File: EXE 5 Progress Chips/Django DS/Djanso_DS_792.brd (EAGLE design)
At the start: 28.9 x 21.9 mm, 1 part

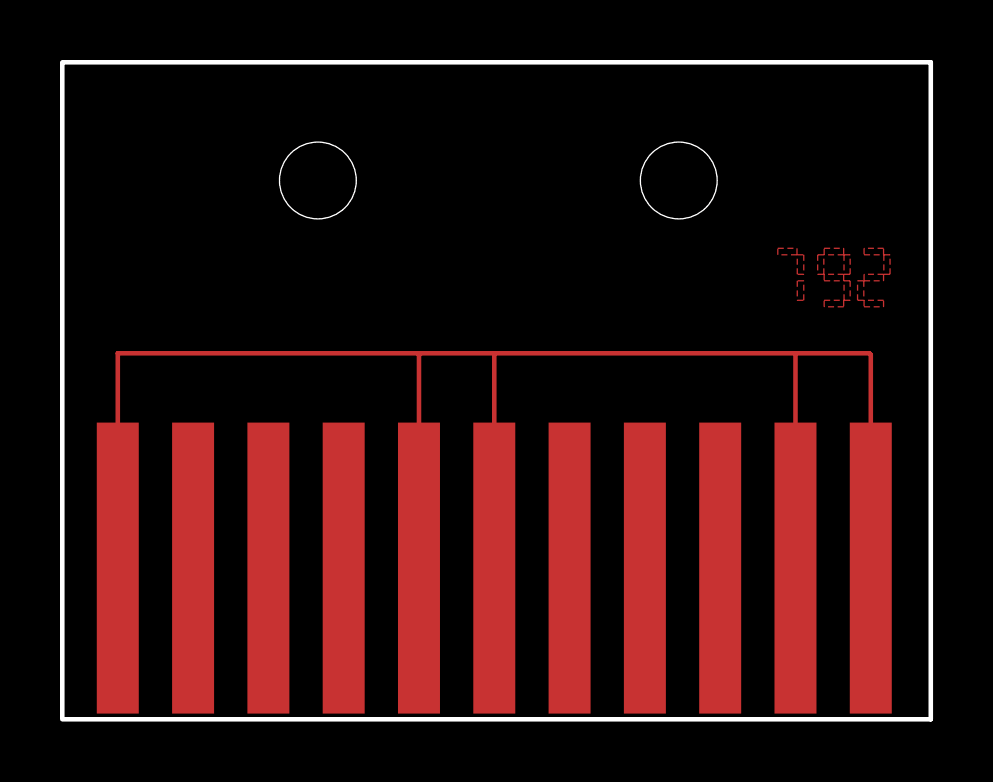
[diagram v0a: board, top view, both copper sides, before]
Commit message: Replace Djanso_DS_792.brd
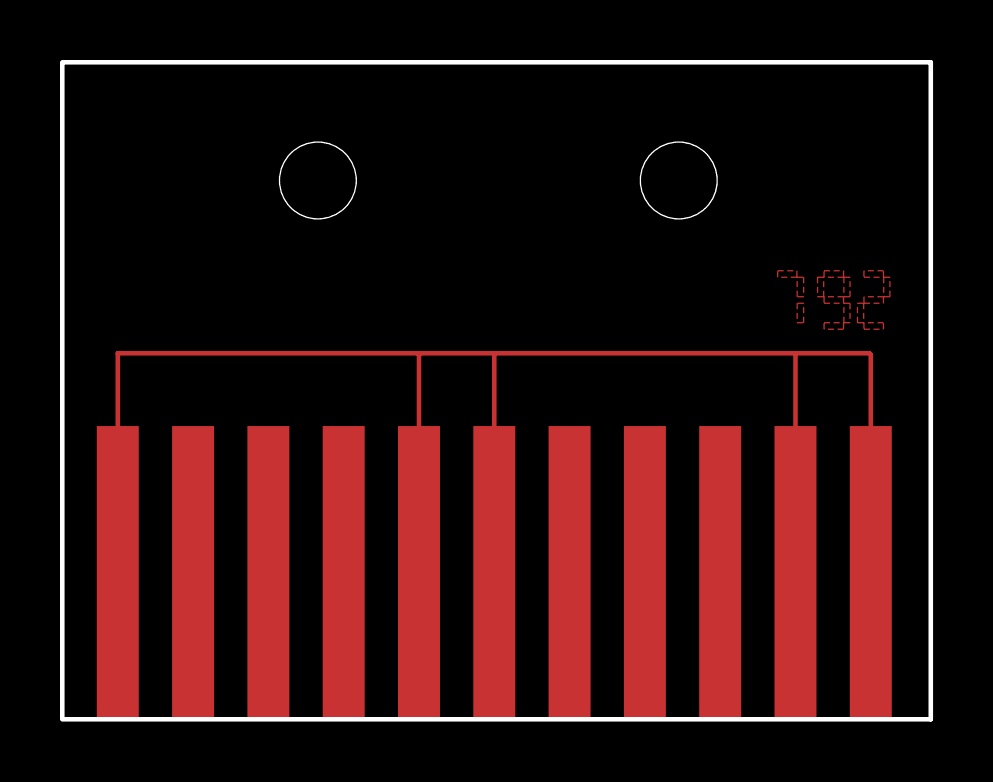
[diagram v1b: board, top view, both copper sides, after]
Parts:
- moved U$1 0.12 mm to (67.3, 20.2)
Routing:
- net N$1: track 60.9 -> 61.5 mm
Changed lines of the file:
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@@
 <setting verticaltext="up"/>
 </settings>
-<grid distance="1" unitdist="mic" unit="mic" style="lines" multiple="1" display="no" altdistance="1" altunitdist="mm" altunit="mm"/>
+<grid distance="1" unitdist="mic" unit="mm" style="lines" multiple="1" display="no" altdistance="1" altunitdist="mm" altunit="mm"/>
 <layers>
 <layer number="1" name="Top" color="4" fill="1" visible="yes" active="yes"/>
@@
 </autorouter>
 <elements>
-<element name="U$1" library="advpins" package="ADCHIP" value="ADVCHIP" x="67.31" y="20.32" smashed="yes"/>
+<element name="U$1" library="advpins" package="ADCHIP" value="ADVCHIP" x="67.31" y="20.205" smashed="yes"/>
 </elements>
 <signals>
@@
 <contactref element="U$1" pad="P$11"/>
 <contactref element="U$1" pad="P$6"/>
-<wire x1="39.7" y1="25.34" x2="39.7" y2="32.5" width="0.1524" layer="1"/>
+<wire x1="39.7" y1="25.225" x2="39.7" y2="32.5" width="0.1524" layer="1"/>
 <wire x1="39.7" y1="32.5" x2="49.8" y2="32.5" width="0.1524" layer="1"/>
 <wire x1="49.8" y1="32.5" x2="52.25" y2="32.5" width="0.1524" layer="1"/>
 <wire x1="52.25" y1="32.5" x2="62.3" y2="32.5" width="0.1524" layer="1"/>
 <wire x1="64.75" y1="32.5" x2="62.3" y2="32.5" width="0.1524" layer="1"/>
-<wire x1="49.74" y1="25.34" x2="49.74" y2="32.44" width="0.1524" layer="1"/>
+<wire x1="49.74" y1="25.225" x2="49.74" y2="32.44" width="0.1524" layer="1"/>
 <wire x1="49.74" y1="32.44" x2="49.8" y2="32.5" width="0.1524" layer="1"/>
-<wire x1="52.25" y1="25.34" x2="52.25" y2="32.5" width="0.1524" layer="1"/>
-<wire x1="62.29" y1="25.34" x2="62.29" y2="32.49" width="0.1524" layer="1"/>
+<wire x1="52.25" y1="25.225" x2="52.25" y2="32.5" width="0.1524" layer="1"/>
+<wire x1="62.29" y1="25.225" x2="62.29" y2="32.49" width="0.1524" layer="1"/>
 <wire x1="62.29" y1="32.49" x2="62.3" y2="32.5" width="0.1524" layer="1"/>
-<wire x1="64.8" y1="25.34" x2="64.8" y2="32.45" width="0.1524" layer="1"/>
+<wire x1="64.8" y1="25.225" x2="64.8" y2="32.45" width="0.1524" layer="1"/>
 <wire x1="64.8" y1="32.45" x2="64.75" y2="32.5" width="0.1524" layer="1"/>
 </signal>
 <signal name="N$4">
-<polygon width="0.001" layer="1">
-<vertex x="62.56625" y="35.132809375"/>
-<vertex x="62.349690625" y="35.132809375"/>
-<vertex x="62.349690625" y="35.7825"/>
-<vertex x="62.56625" y="35.7825"/>
+<polygon width="0.001" layer="1" rank="4">
+<vertex x="62.56225" y="34.384809375"/>
+<vertex x="62.345690625" y="34.384809375"/>
+<vertex x="62.345690625" y="35.0345"/>
+<vertex x="62.56225" y="35.0345"/>
 </polygon>
 </signal>
 <signal name="N$2">
-<polygon width="0.001" layer="1">
-<vertex x="62.340690625" y="35.7825"/>
-<vertex x="61.7" y="35.7825"/>
-<vertex x="61.7" y="35.999059375"/>
-<vertex x="62.340690625" y="35.999059375"/>
+<polygon width="0.001" layer="1" rank="4">
+<vertex x="62.336690625" y="35.0345"/>
+<vertex x="61.696" y="35.0345"/>
+<vertex x="61.696" y="35.251059375"/>
+<vertex x="62.336690625" y="35.251059375"/>
 </polygon>
 </signal>
 <signal name="N$3">
-<polygon width="0.001" layer="1">
-<vertex x="62.349690625" y="34.91625"/>
-<vertex x="62.349690625" y="34.266559375"/>
-<vertex x="62.56625" y="34.266559375"/>
-<vertex x="62.56625" y="34.91625"/>
+<polygon width="0.001" layer="1" rank="4">
+<vertex x="62.345690625" y="34.16825"/>
+<vertex x="62.345690625" y="33.518559375"/>
+<vertex x="62.56225" y="33.518559375"/>
+<vertex x="62.56225" y="34.16825"/>
 </polygon>
 </signal>
 <signal name="N$10">
-<polygon width="0.001" layer="1">
-<vertex x="63.246259375" y="35.132809375"/>
-<vertex x="63.246259375" y="34.91625"/>
-<vertex x="63.895940625" y="34.91625"/>
-<vertex x="63.895940625" y="35.132809375"/>
+<polygon width="0.001" layer="1" rank="4">
+<vertex x="63.242259375" y="34.384809375"/>
+<vertex x="63.242259375" y="34.16825"/>
+<vertex x="63.891940625" y="34.16825"/>
+<vertex x="63.891940625" y="34.384809375"/>
 </polygon>
 </signal>
 <signal name="N$14">
-<polygon width="0.001" layer="1">
-<vertex x="63.895940625" y="34.05"/>
-<vertex x="63.246259375" y="34.05"/>
-<vertex x="63.246259375" y="34.266559375"/>
-<vertex x="63.895940625" y="34.266559375"/>
+<polygon width="0.001" layer="1" rank="4">
+<vertex x="63.891940625" y="33.302"/>
+<vertex x="63.242259375" y="33.302"/>
+<vertex x="63.242259375" y="33.518559375"/>
+<vertex x="63.891940625" y="33.518559375"/>
 </polygon>
 </signal>
 <signal name="N$9">
-<polygon width="0.001" layer="1">
-<vertex x="64.112509375" y="34.266559375"/>
-<vertex x="63.907940625" y="34.266559375"/>
-<vertex x="63.907940625" y="34.91625"/>
-<vertex x="64.112509375" y="34.91625"/>
+<polygon width="0.001" layer="1" rank="4">
+<vertex x="64.108509375" y="33.518559375"/>
+<vertex x="63.903940625" y="33.518559375"/>
+<vertex x="63.903940625" y="34.16825"/>
+<vertex x="64.108509375" y="34.16825"/>
 </polygon>
 </signal>
 <signal name="N$8">
-<polygon width="0.001" layer="1">
-<vertex x="63.906940625" y="35.7825"/>
-<vertex x="63.906940625" y="35.132809375"/>
-<vertex x="64.112509375" y="35.132809375"/>
-<vertex x="64.112509375" y="35.7825"/>
+<polygon width="0.001" layer="1" rank="4">
+<vertex x="63.902940625" y="35.0345"/>
+<vertex x="63.902940625" y="34.384809375"/>
+<vertex x="64.108509375" y="34.384809375"/>
+<vertex x="64.108509375" y="35.0345"/>
 </polygon>
 </signal>
 <signal name="N$6">
-<polygon width="0.001" layer="1">
-<vertex x="63.029690625" y="35.7825"/>
-<vertex x="63.029690625" y="35.132809375"/>
-<vertex x="63.234259375" y="35.132809375"/>
-<vertex x="63.234259375" y="35.7825"/>
+<polygon width="0.001" layer="1" rank="4">
+<vertex x="63.025690625" y="35.0345"/>
+<vertex x="63.025690625" y="34.384809375"/>
+<vertex x="63.230259375" y="34.384809375"/>
+<vertex x="63.230259375" y="35.0345"/>
 </polygon>
 </signal>
 <signal name="N$5">
-<polygon width="0.001" layer="1">
-<vertex x="63.895940625" y="35.7825"/>
-<vertex x="63.246259375" y="35.7825"/>
-<vertex x="63.246259375" y="35.999059375"/>
-<vertex x="63.895940625" y="35.999059375"/>
+<polygon width="0.001" layer="1" rank="4">
+<vertex x="63.891940625" y="35.0345"/>
+<vertex x="63.242259375" y="35.0345"/>
+<vertex x="63.242259375" y="35.251059375"/>
+<vertex x="63.891940625" y="35.251059375"/>
 </polygon>
 </signal>
 <signal name="N$15">
-<polygon width="0.001" layer="1">
-<vertex x="64.57595" y="34.266559375"/>
-<vertex x="64.57595" y="34.05"/>
-<vertex x="65.225640625" y="34.05"/>
-<vertex x="65.225640625" y="34.266559375"/>
+<polygon width="0.001" layer="1" rank="4">
+<vertex x="64.57195" y="33.518559375"/>
+<vertex x="64.57195" y="33.302"/>
+<vertex x="65.221640625" y="33.302"/>
+<vertex x="65.221640625" y="33.518559375"/>
 </polygon>
 </signal>
 <signal name="N$11">
-<polygon width="0.001" layer="1">
-<vertex x="64.56695" y="34.266559375"/>
-<vertex x="64.359390625" y="34.266559375"/>
-<vertex x="64.359390625" y="34.91625"/>
-<vertex x="64.56695" y="34.91625"/>
+<polygon width="0.001" layer="1" rank="4">
+<vertex x="64.56295" y="33.518559375"/>
+<vertex x="64.355390625" y="33.518559375"/>
+<vertex x="64.355390625" y="34.16825"/>
+<vertex x="64.56295" y="34.16825"/>
 </polygon>
 </signal>
 <signal name="N$12">
-<polygon width="0.001" layer="1">
-<vertex x="64.57595" y="35.132809375"/>
-<vertex x="64.57595" y="34.91625"/>
-<vertex x="65.225640625" y="34.91625"/>
-<vertex x="65.225640625" y="35.132809375"/>
+<polygon width="0.001" layer="1" rank="4">
+<vertex x="64.57195" y="34.384809375"/>
+<vertex x="64.57195" y="34.16825"/>
+<vertex x="65.221640625" y="34.16825"/>
+<vertex x="65.221640625" y="34.384809375"/>
 </polygon>
 </signal>
 <signal name="N$13">
-<polygon width="0.001" layer="1">
-<vertex x="65.234640625" y="35.7825"/>
-<vertex x="65.234640625" y="35.132809375"/>
-<vertex x="65.4422" y="35.132809375"/>
-<vertex x="65.4422" y="35.7825"/>
+<polygon width="0.001" layer="1" rank="4">
+<vertex x="65.230640625" y="35.0345"/>
+<vertex x="65.230640625" y="34.384809375"/>
+<vertex x="65.4382" y="34.384809375"/>
+<vertex x="65.4382" y="35.0345"/>
 </polygon>
 </signal>
 <signal name="N$7">
-<polygon width="0.001" layer="1">
-<vertex x="64.57595" y="35.999059375"/>
-<vertex x="64.57595" y="35.7825"/>
-<vertex x="65.225640625" y="35.7825"/>
-<vertex x="65.225640625" y="35.999059375"/>
-</polygon>
-</signal>
+<polygon width="0.001" layer="1" rank="4">
+<vertex x="64.57195" y="35.251059375"/>
+<vertex x="64.57195" y="35.0345"/>
+<vertex x="65.221640625" y="35.0345"/>
+<vertex x="65.221640625" y="35.251059375"/>
+</polygon>
+</signal>
